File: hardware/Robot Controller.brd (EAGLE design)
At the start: 50.5 x 51.4 mm, 11 parts

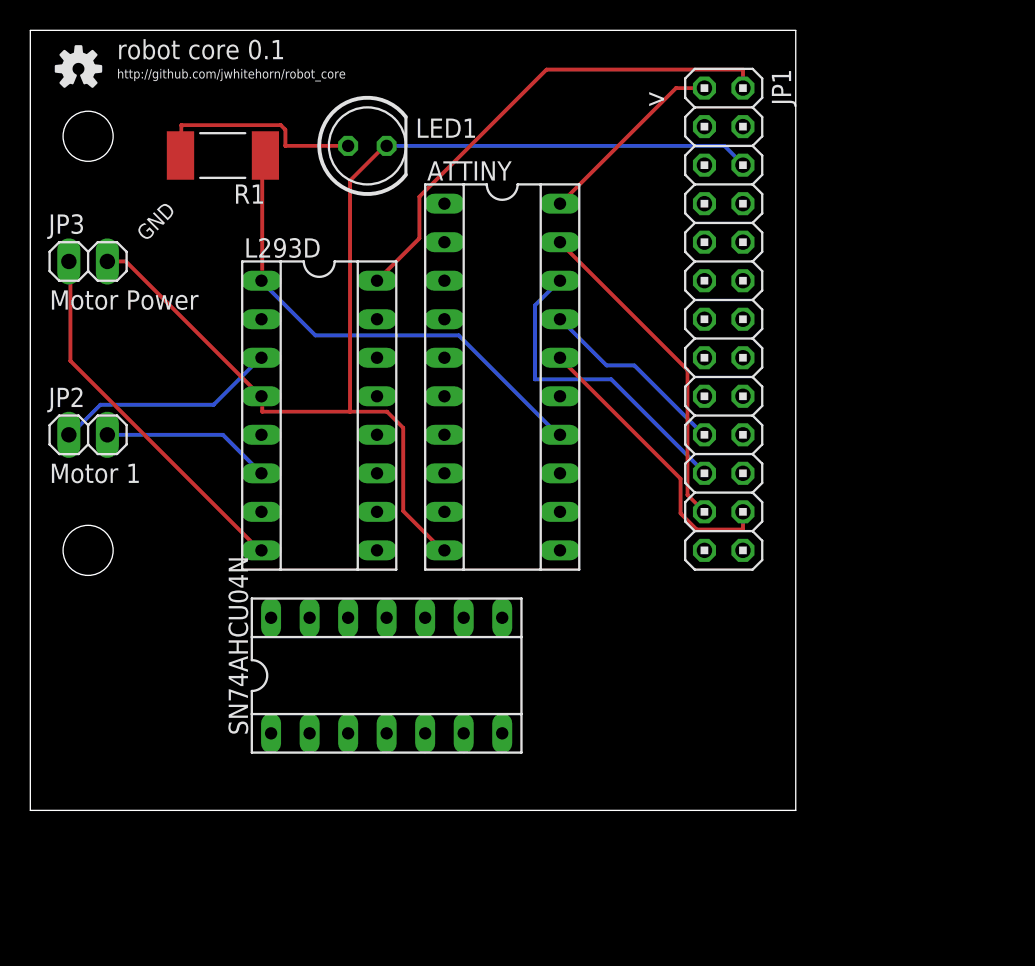
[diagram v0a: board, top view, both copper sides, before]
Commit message: tweak hardware design
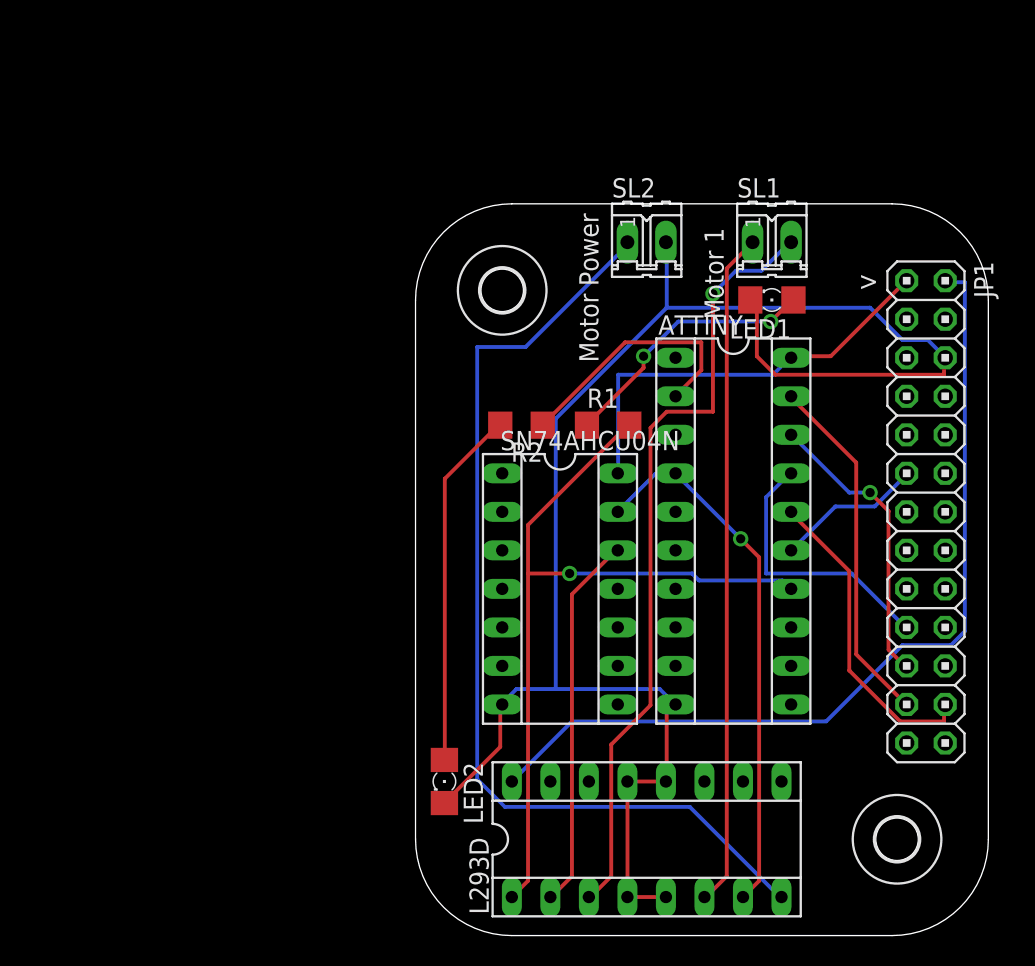
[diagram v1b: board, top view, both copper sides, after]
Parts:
- removed JP2: Motor 1, pinhead:1X02
- removed JP3: Motor Power, pinhead:1X02
- removed U$1, U$2: (no value), SparkFun-Electromechanical:STAND-OFF
- removed U$4: (no value), SparkFun-Aesthetics:OSHW-LOGO-S
- added H1, H2: MOUNT-HOLE2.8, holes:2,8
- added LED2: (no value), led:1206
- added R2: (no value), resistor:R3216
- added SL1, SL2: (no value), con-amp-quick:02P
- LED1: device led:LED5MM -> led:1206
- R1: device resistor:R6332 -> resistor:R3216
- moved L293D 35.3 mm to (77.5, 26.7), turned to 0 degrees
- moved R1 31.0 mm to (74.9, 54.0), turned to 0 degrees
- moved LED1 28.5 mm to (85.7, 62.2), turned to 180 degrees
- moved JP1 18.4 mm to (95.9, 48.3)
- moved ATTINY 18.3 mm to (83.2, 47.0)
- moved SN74AHCU04N 12.8 mm to (71.8, 43.2), turned to 270 degrees
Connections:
- removed net N$11: LED1.A, R1.2
- new net N$16: ATTINY.2, R2.1
- new net N$17: LED2.A, R2.2
- new net N$3: LED1.A, R1.1
- net GND: now also LED1.C, LED2.C, SL2.2; no longer JP3.2, LED1.K
- net N$1: now also R1.2; no longer R1.1
- net N$10: now also SL2.1; no longer JP3.1
- net N$8: now also SL1.2; no longer JP2.1
- net N$9: now also SL1.1; no longer JP2.2
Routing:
- net N$10: track 24.4 -> 64.7 mm
- net N$8: track 14.8 -> 51.6 mm, vias 0 -> 1
- net N$13: track 0.00 -> 35.5 mm, vias 0 -> 1
- net N$9: track 11.2 -> 44.6 mm
- net GND: track 76.5 -> 108.7 mm
- net N$12: track 32.7 -> 58.3 mm
- net N$15: track 0.00 -> 24.8 mm
- net N$17: track 0.00 -> 23.7 mm
- net N$1: track 32.3 -> 52.1 mm, vias 0 -> 1
- net N$3: track 0.00 -> 17.5 mm, vias 0 -> 2
- net N$16: track 0.00 -> 17.0 mm
- net VCC: track 12.7 -> 28.1 mm
- net N$11: track 14.2 -> 0.00 mm
- net N$2: track 0.00 -> 9.79 mm
- net N$5: track 12.7 -> 18.1 mm
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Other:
- board size 50.5 x 51.4 mm -> 37.8 x 48.2 mm
- board text added: "robot core"
- board text removed: "GND"
- board text removed: "http://github.com/jwhitehorn/robot_core"
- board text removed: "robot core 0.1"
